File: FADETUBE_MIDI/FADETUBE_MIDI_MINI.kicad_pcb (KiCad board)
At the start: 2 copper layers, 70 x 70 mm, 15 parts, among them J1_DECK_A1 B8B-PH-K-S, J2_DECK_B1 B8B-PH-K-S

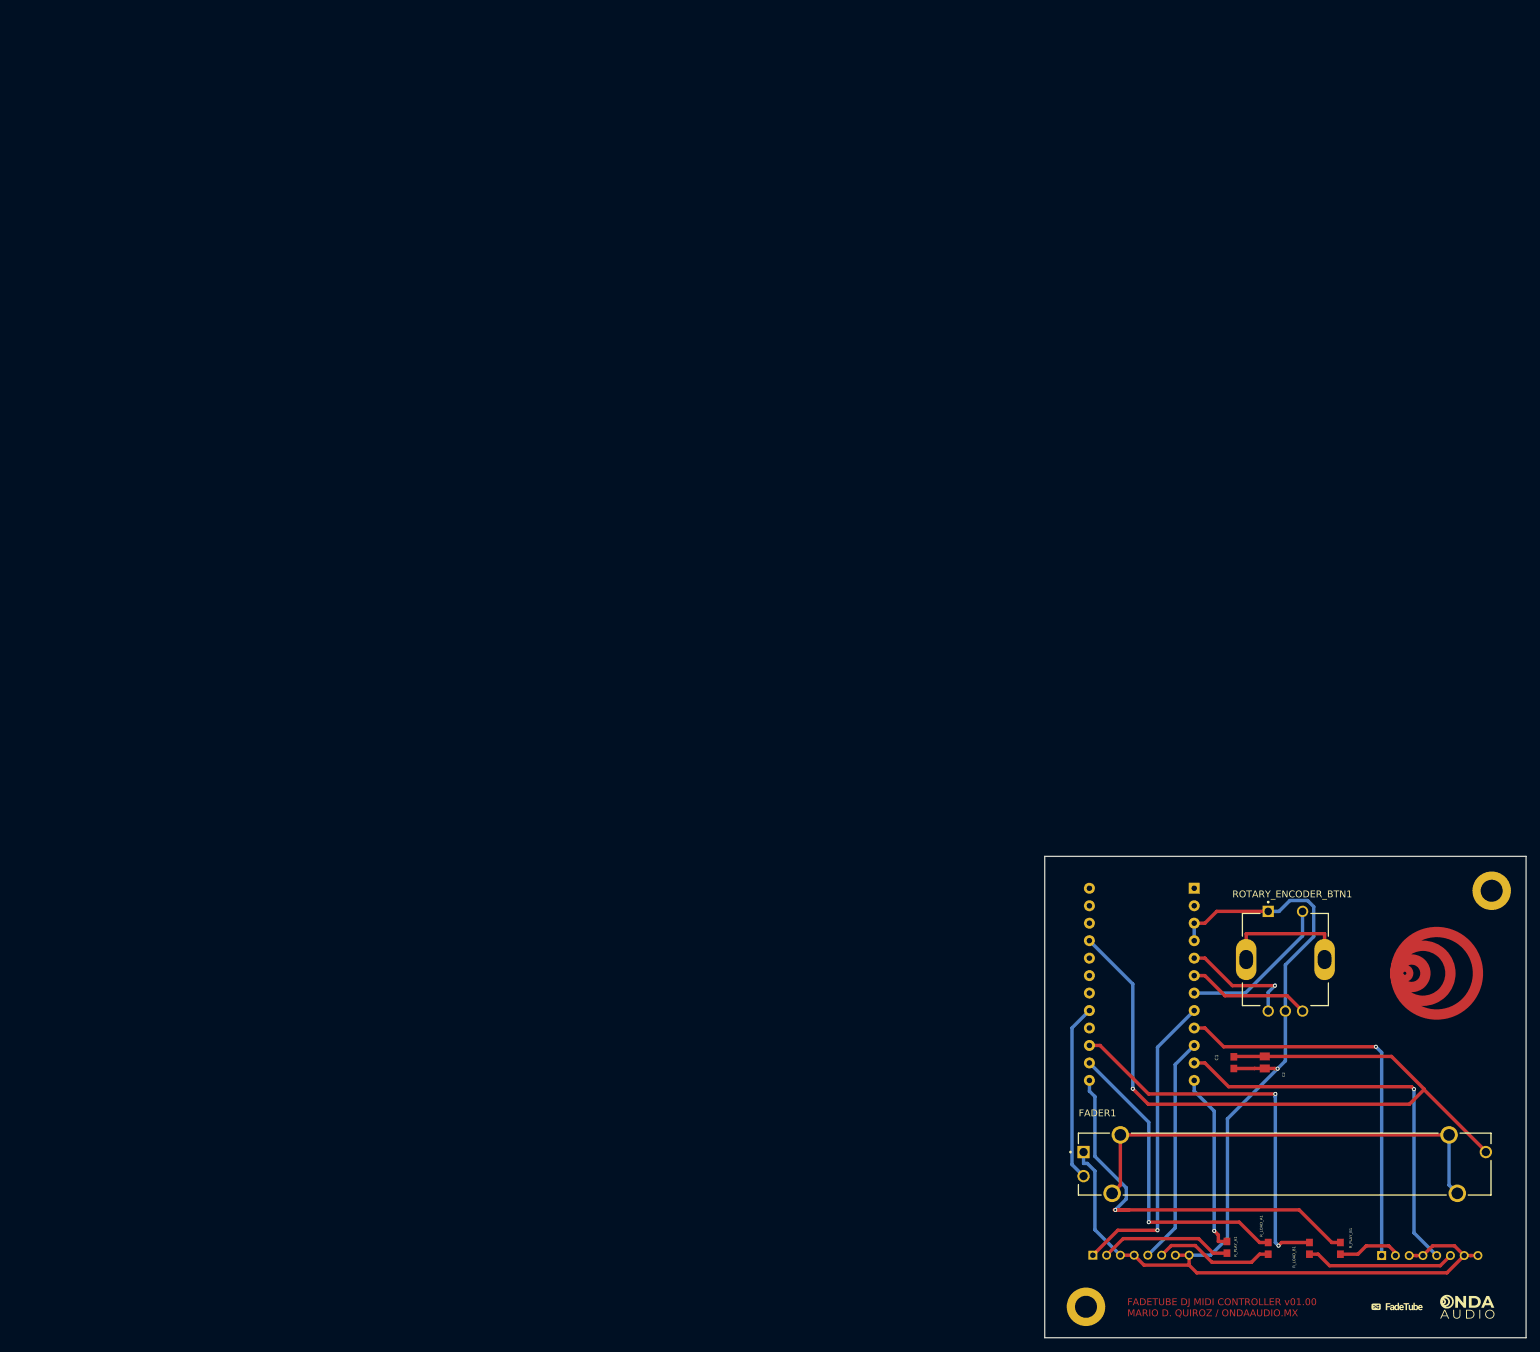
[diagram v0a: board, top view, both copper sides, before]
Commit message: new updates
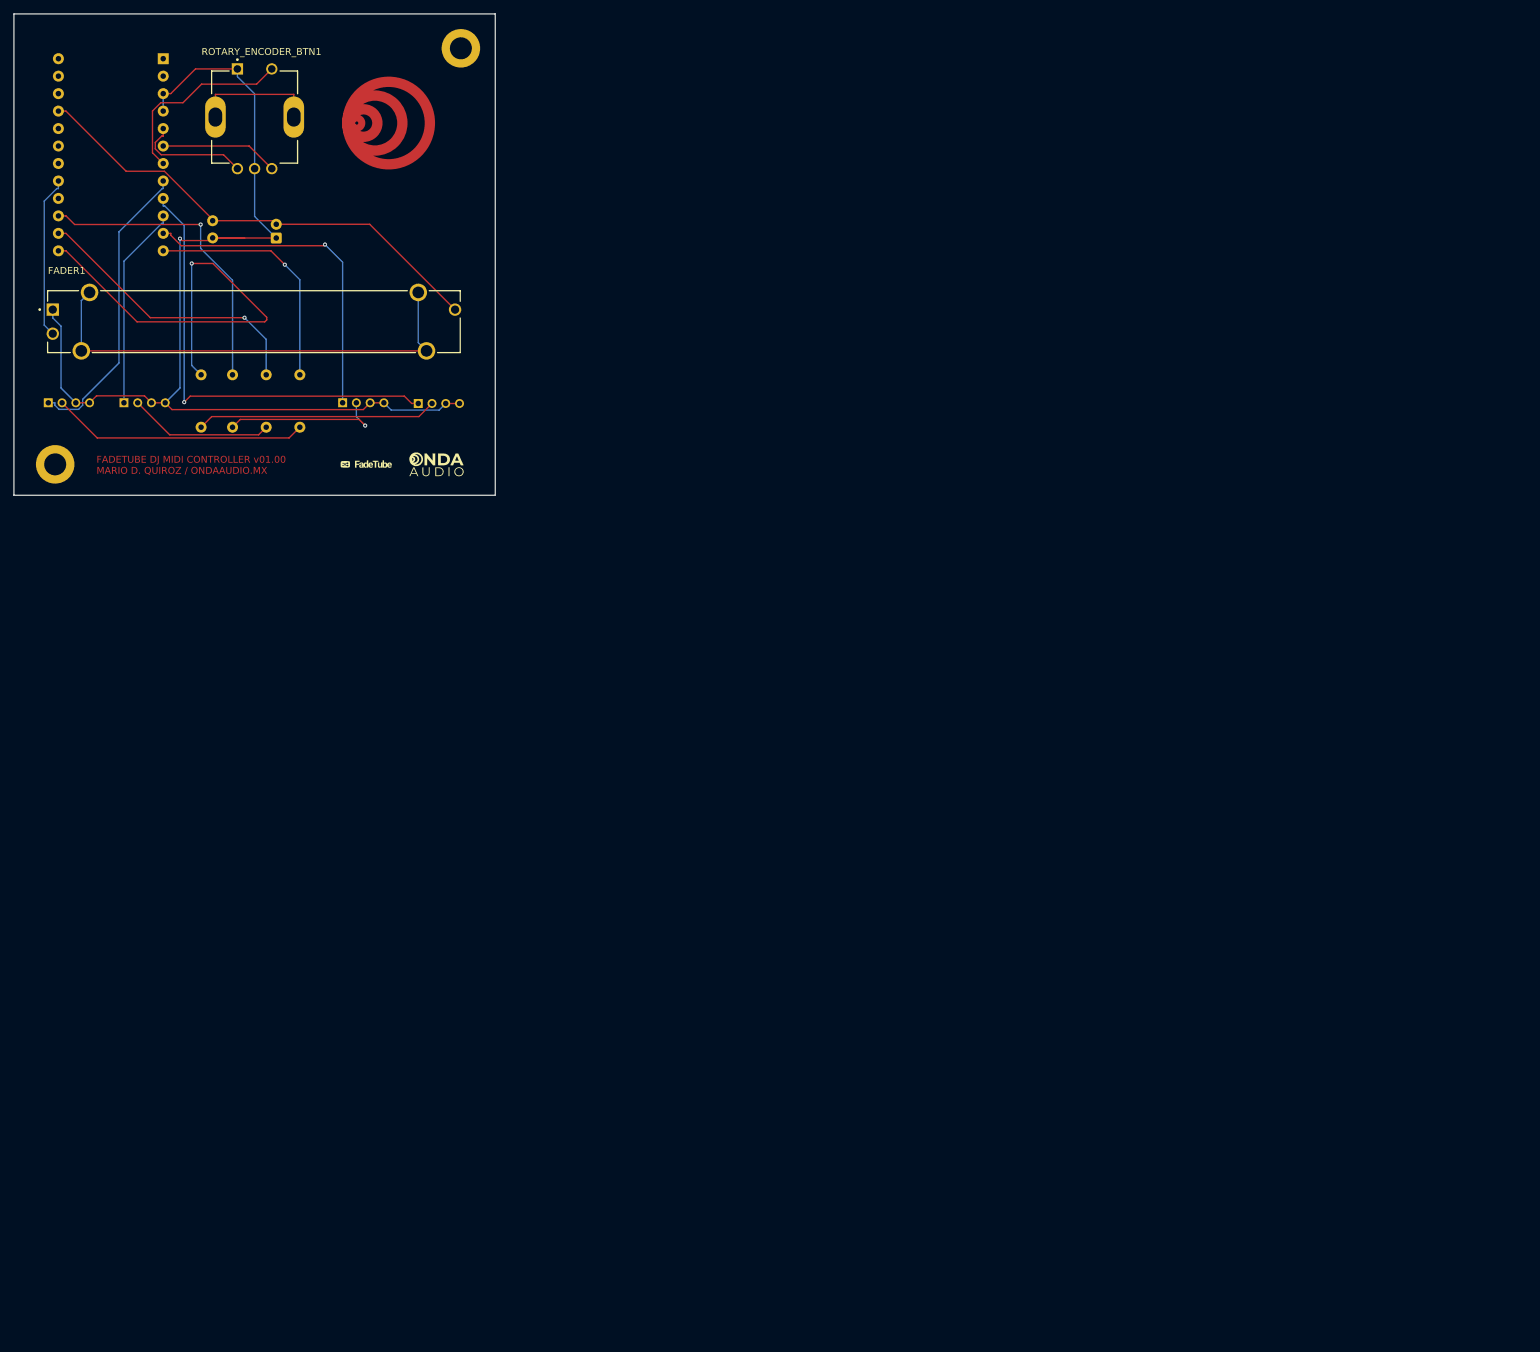
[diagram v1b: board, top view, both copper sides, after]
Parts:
- removed J1_DECK_A1, J2_DECK_B1: B8B-PH-K-S, FADETUBE_LIBRARY:JST_B8B-PH-K-S
- added JPH_DECK_A1: B4B-PH-K-S, FADETUBE_LIBRARY:JST_B4B-PH-K-S, B.Cu at (-26.9, 18.5)
- added JPH_DECK_A2: B4B-PH-K-S, FADETUBE_LIBRARY:JST_B4B-PH-K-S, B.Cu at (-15.9, 18.5)
- added JPH_DECK_B3: B4B-PH-K-S, FADETUBE_LIBRARY:JST_B4B-PH-K-S, B.Cu at (26.9, 18.6)
- added JPH_DECK_B4: B4B-PH-K-S, FADETUBE_LIBRARY:JST_B4B-PH-K-S, B.Cu at (15.9, 18.5)
- C1: footprint FADETUBE_LIBRARY:CAPC1608X90 -> Capacitor_THT:C_Disc_D3.0mm_W1.6mm_P2.50mm; moved to B.Cu
- C2: footprint FADETUBE_LIBRARY:CAPC2012X88N -> Capacitor_THT:CP_Radial_D5.0mm_P2.00mm; moved to B.Cu
- R_LOAD_A1, R_LOAD_B1, R_PLAY_A1, R_PLAY_B1: footprint FADETUBE_LIBRARY:RESC1608X55 -> Resistor_THT:R_Axial_DIN0207_L6.3mm_D2.5mm_P7.62mm_Horizontal; moved to B.Cu
- moved R_PLAY_B1 204.2 mm to (-7.68, 22.6)
- moved R_LOAD_B1 196.9 mm to (-3.11, 22.6)
- moved FADER1 193.6 mm to (0.00, 7.24)
- moved FADETUBE-LOGO 193.6 mm to (16.1, 28.0)
- moved MH2 193.6 mm to (-28.9, 28.0)
- moved ONDAAUDIO-LOGO 193.6 mm to (26.6, 28.0)
- moved ROTARY_ENCODER_BTN1 193.6 mm to (0.10, -22.5)
- moved MH1 193.6 mm to (30.1, -32.5)
- moved ArduinoProMicroATmega32U4USBC-1 192.4 mm to (-28.4, -3.06)
- moved C1 190.9 mm to (-6.00, -4.94)
- moved R_LOAD_A1 188.4 mm to (1.79, 22.6)
- moved C2 187.2 mm to (3.25, -4.92)
- moved R_PLAY_A1 180.0 mm to (6.68, 22.6)
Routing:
- net Net-(ArduinoProMicroATmega32U4USBC-1-VCC): track 110.9 -> 69.7 mm, vias 1 -> 0
- net Net-(JPH_DECK_B3-Pad2): track 9.34 -> 35.0 mm
- net Net-(JPH_DECK_A1-Pad2): track 19.4 -> 37.3 mm
- net GND: track 172.3 -> 158.7 mm
- net Net-(ArduinoProMicroATmega32U4USBC-1-D14): track 57.8 -> 45.0 mm, vias 2 -> 1
- net Net-(ArduinoProMicroATmega32U4USBC-1-D8/A8): track 59.1 -> 48.6 mm
- net Net-(ArduinoProMicroATmega32U4USBC-1-~D9/A9): track 26.1 -> 35.4 mm
- net Net-(ArduinoProMicroATmega32U4USBC-1-~D6/A7): track 58.3 -> 65.9 mm
- net Net-(ArduinoProMicroATmega32U4USBC-1-D4/A6): track 22.8 -> 28.2 mm
- net Net-(ArduinoProMicroATmega32U4USBC-1-D7): track 33.3 -> 29.7 mm
- net Net-(ArduinoProMicroATmega32U4USBC-1-D16): track 45.3 -> 41.8 mm
- net Net-(JPH_DECK_A2-Pad2): track 17.6 -> 21.1 mm
- net Net-(FADER1-SHIELD-PadSH1): track 65.8 -> 68.2 mm
- net Net-(JPH_DECK_B4-Pad2): track 21.8 -> 24.0 mm, vias 0 -> 1
- net Net-(ArduinoProMicroATmega32U4USBC-1-D18/A0): track 25.8 -> 23.7 mm
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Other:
- board text added: "1 - PLAY A BTN"
- board text added: "1 - PLAY B BTN"
- board text added: "2 - PLAY A LED"
- board text added: "2 - PLAY B LED"
- board text added: "3 - PLAY A LED GND"
- board text added: "3 - PLAY B LED GND"
- board text added: "4 - PLAY A BTN GRND"
- board text added: "4 - PLAY B BTN GRND"
- board text added: "5 - LOAD A BTN"
- board text added: "5 - LOAD B BTN"
- board text added: "6 - LOAD A BTN LED"
- board text added: "6 - LOAD B BTN LED"
- board text added: "7 - LOAD A LED GND"
- board text added: "7 - LOAD B LED GND"
- board text added: "8 - LOAD A BTN GRND"
- board text added: "8 - LOAD B BTN GRND"
- board text added: "__.-{dblquote}..--,__ __..---{dblquote} | _| {dblquote}-_\ __.---{dblquote} | V|::.-{dblquote}-._D _--{dblquote}{dblquote}.-.._ ,,::::::'{dblquote}\/{dblquote}{dblquote}'-:-:/ _.-{dblquote}{dblquote}::_:_:::::'-8b---{dblquote} {dblquote}' .-/ ::::< |\::::::{dblquote}\ \/:::/::::'\\ |:::b::\ /|::/:::/::::-::b:%b:\| \/::::d:|8:::b:{dblquote}%%%%%\ |\:b:dP:d.:::%%%%%{dblquote}{dblquote}{dblquote}-, 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"
- board text added: "{dblquote}This circuit dreams in harmonics{dblquote} (.◕‿‿◕.)"
